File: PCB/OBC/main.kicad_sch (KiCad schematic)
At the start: 33 parts, among them J7 USB_C_Receptacle_USB2.0_16P, U2 STM32F405RGTx, U5 USBLC6-2SC6

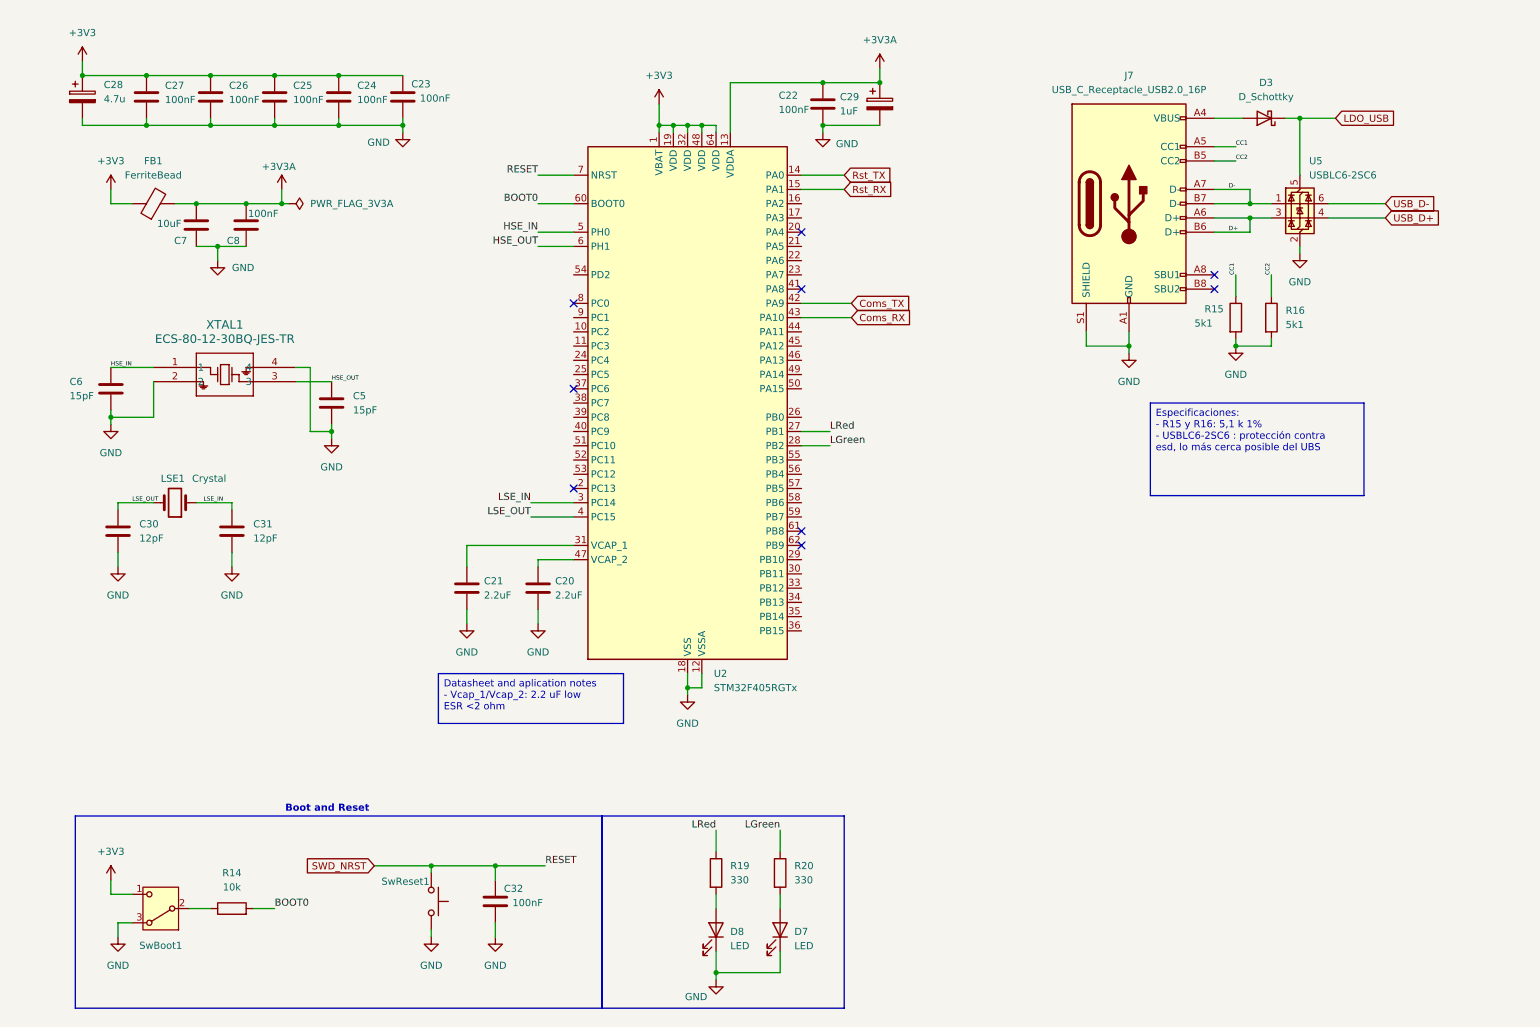
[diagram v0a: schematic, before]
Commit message: Watchdog
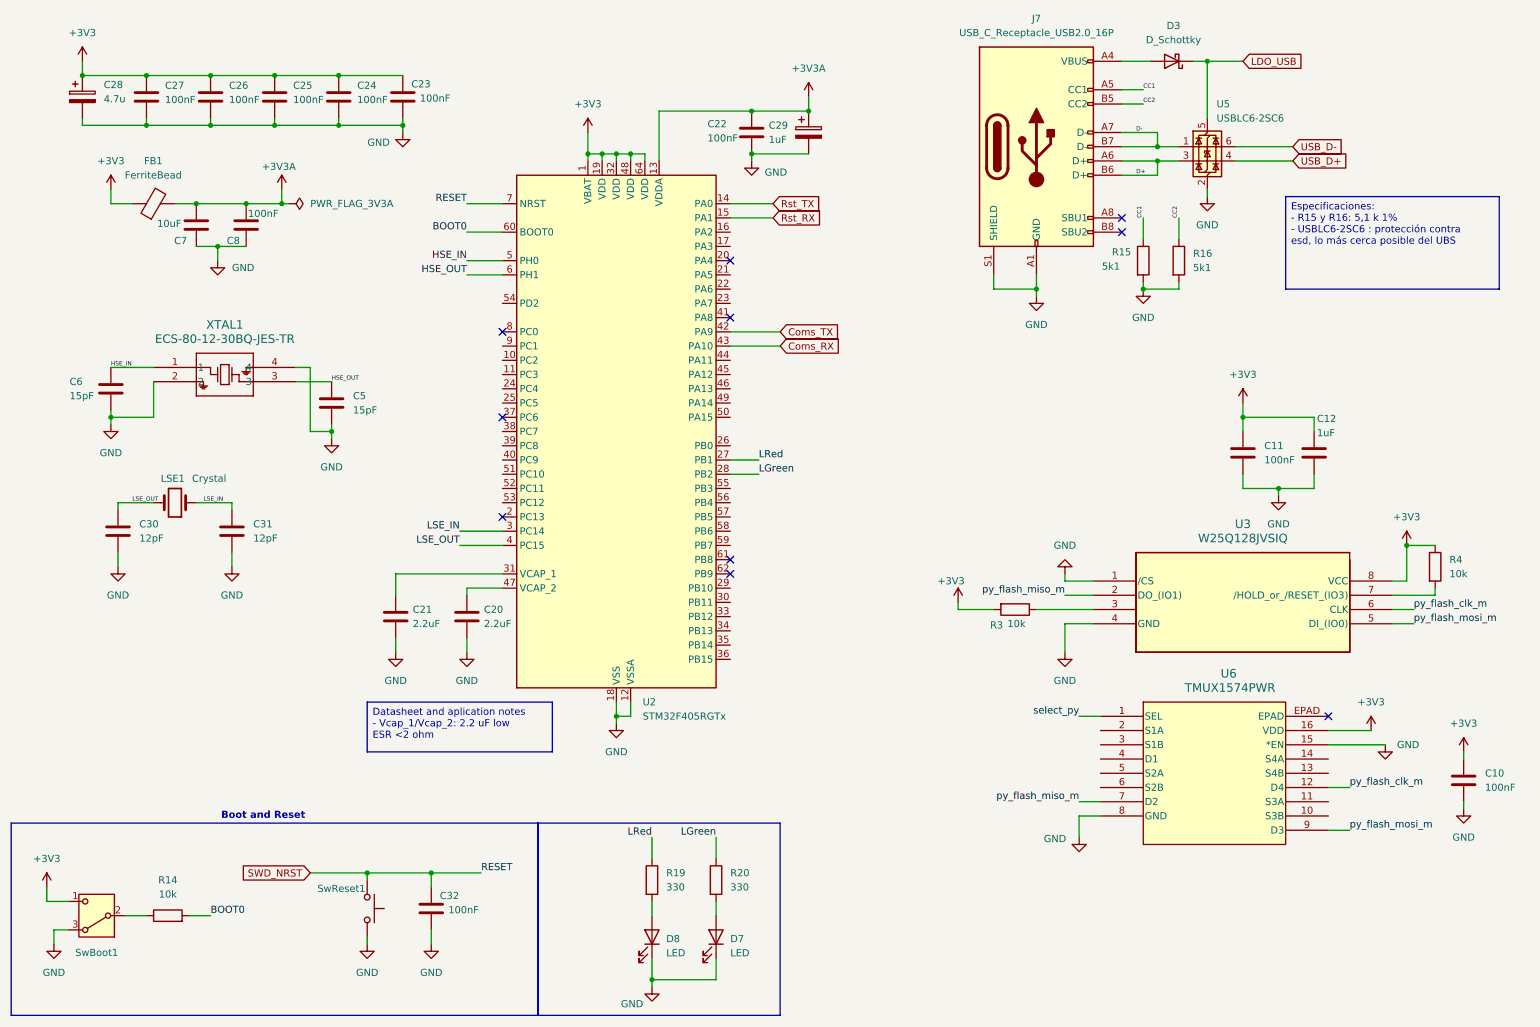
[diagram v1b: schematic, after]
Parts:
- added C10, C11: 100nF, symbol Device:C
- added C12: 1uF, symbol Device:C
- added R3, R4: 10k, symbol Device:R
- added U3: W25Q128JVSIQ, SOIC_128JVSIQ_WIN, symbol W25Q128JVSIQ:W25Q128JVSIQ
- added U6: TMUX1574PWR, PWP16_2P31X2P46_TEX, symbol TMUX1574PWR:TMUX1574PWR
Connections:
- net +3V3: now also C10.1, C11.1, C12.1, R3.2, R4.1, U3.8 (VCC), U6.16 (VDD)
- net GND: now also C10.2, C11.2, C12.2, U3.1 (/CS), U3.4 (GND), U6.15 (*EN), U6.8 (GND)
- new net: R3.1, U3.3
- new net: R4.2, U3.7 (/HOLD_or_/RESET_(IO3))
- new net py_flash_clk_m: U3.6 (CLK), U6.12 (D4)
- new net py_flash_miso_m: U3.2 (DO_(IO1)), U6.7 (D2)
- new net py_flash_mosi_m: U3.5 (DI_(IO0)), U6.9 (D3)
- new net select_py: U6.1 (SEL)
- no-connect marks 9 -> 10
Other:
- moved on the sheet: C20, C21, C22, C29, C32, D3, D7, D8, J7, R14, R15, R16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
